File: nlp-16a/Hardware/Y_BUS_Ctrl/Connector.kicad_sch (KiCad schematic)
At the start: 62 parts, among them J1 Conn_02x20_Odd_Even, J2 Conn_02x20_Odd_Even, J3 Conn_02x10_Odd_Even, J4 Conn_02x10_Counter_Clockwise, J5 Screw_Terminal_01x02

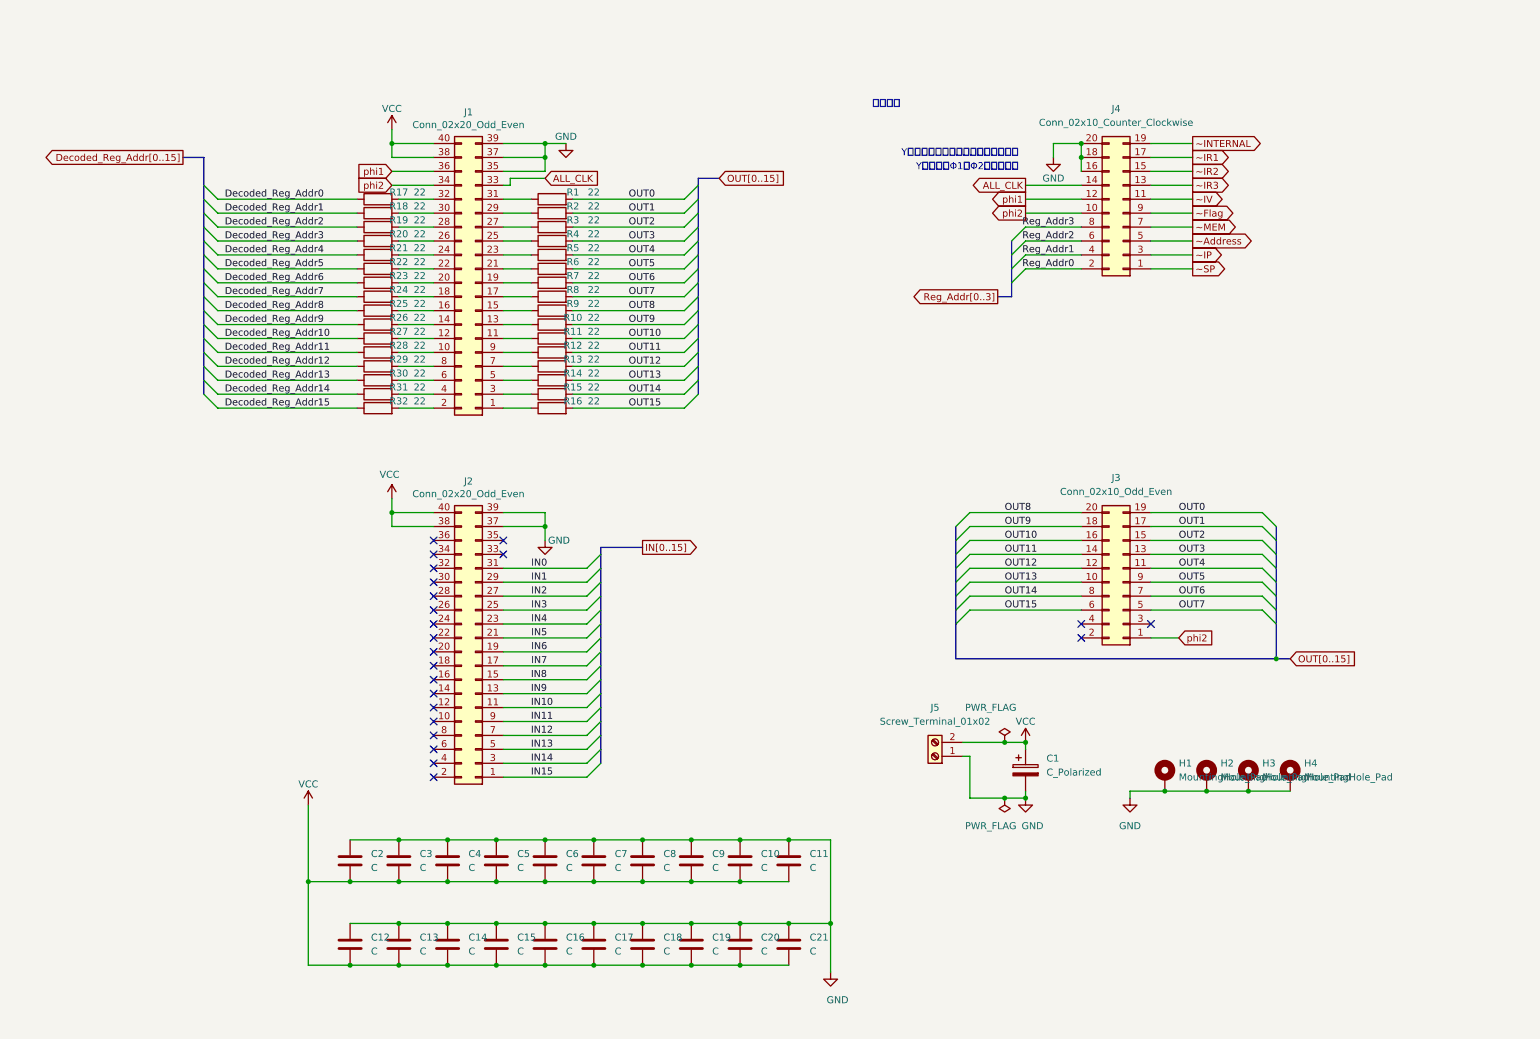
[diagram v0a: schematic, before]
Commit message: Y-BUS制御完成
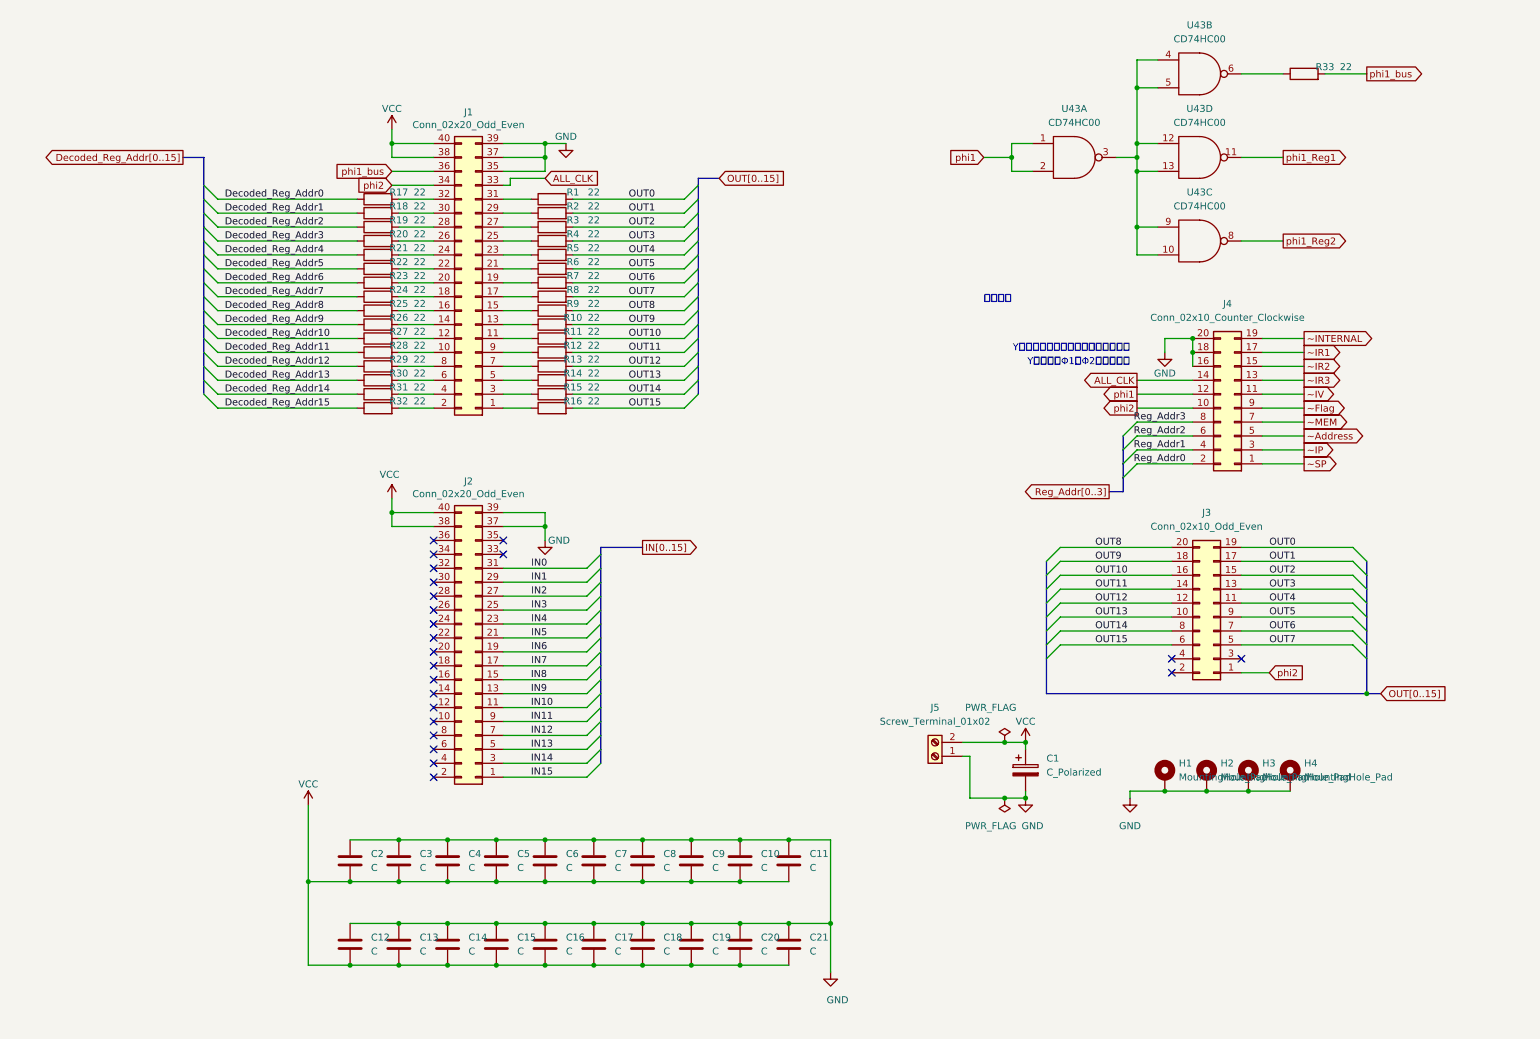
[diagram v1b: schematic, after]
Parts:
- added R33: 22, Resistor_SMD:R_0603_1608Metric_Pad0.98x0.95mm_HandSolder, symbol Device:R
- added U43: CD74HC00, Package_DIP:DIP-14_W7.62mm, symbol CD74HCXX:CD74HC00
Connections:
- net GND: now also U43.7 (GND), U43.7 (GND), U43.7 (GND), U43.7 (GND)
- net VCC: now also U43.14 (VCC), U43.14 (VCC), U43.14 (VCC), U43.14 (VCC)
- net phi1: now also U43.1, U43.2; no longer J1.36 (Pin_36)
- new net: U43.10, U43.12, U43.13, U43.3, U43.4, U43.5, U43.9
- new net: R33.1, U43.6
- new net phi1_Reg1: U43.11
- new net phi1_Reg2: U43.8
- new net phi1_bus: J1.36 (Pin_36), R33.2
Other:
- moved on the sheet: J3, J4

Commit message: Y BUS制御 更新
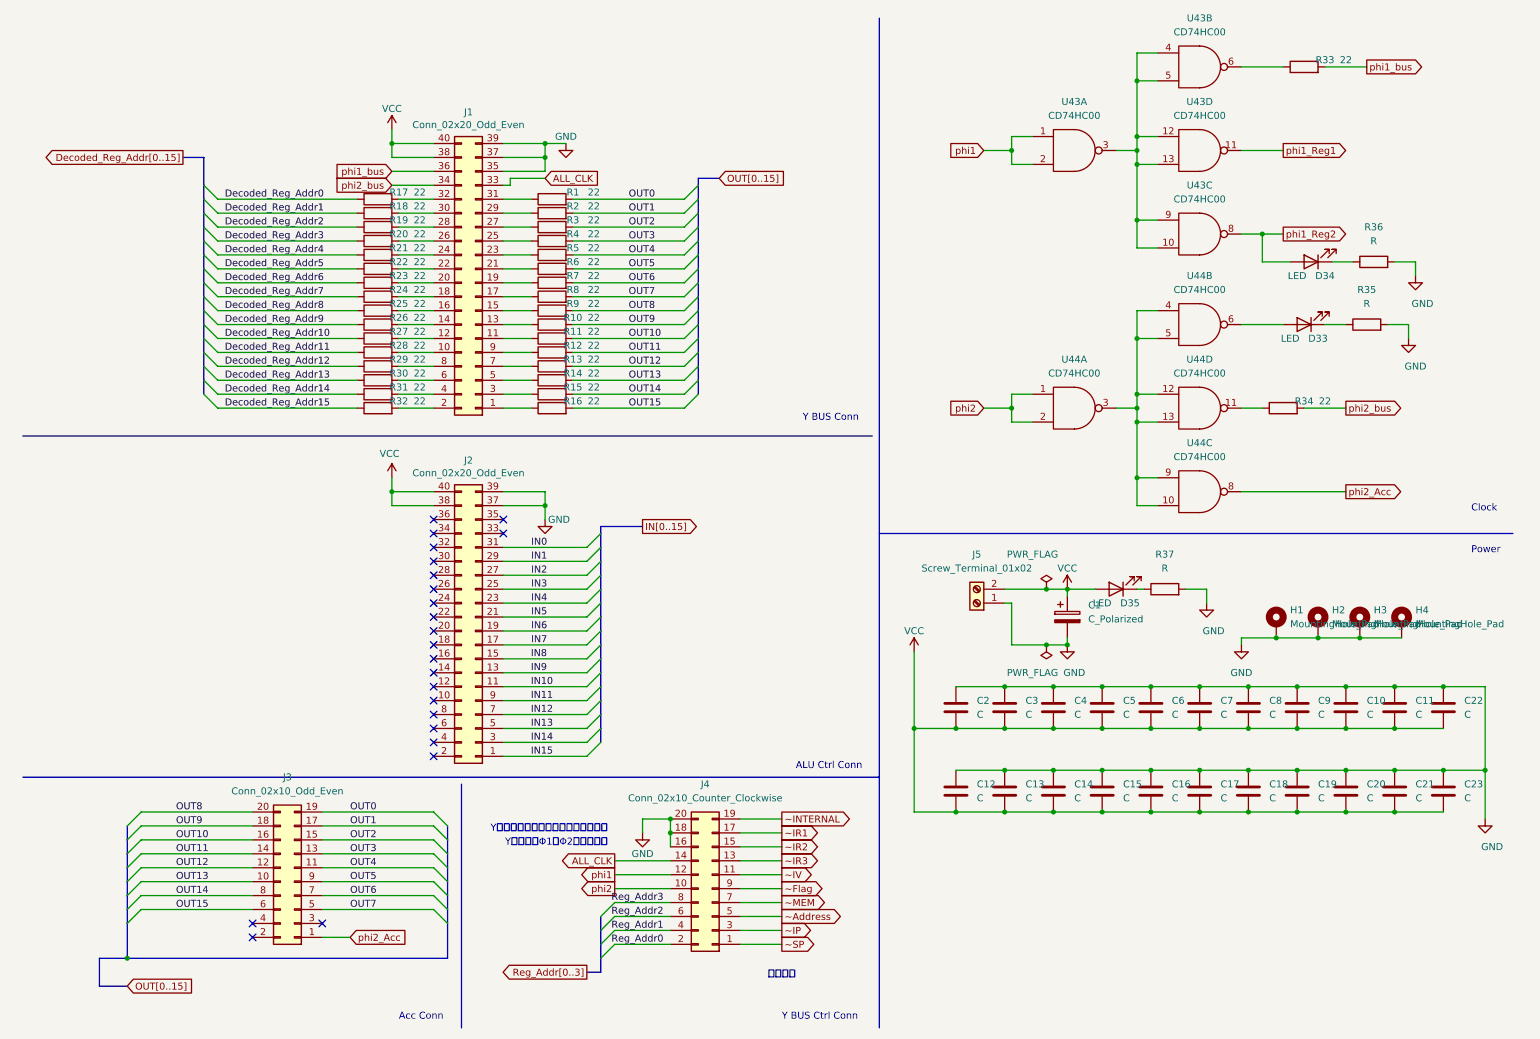
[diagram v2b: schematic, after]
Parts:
- added C22, C23: C, Capacitor_THT:C_Disc_D7.5mm_W2.5mm_P5.00mm, symbol Device:C
- added D33, D34, D35: LED, LED_THT:LED_D3.0mm, symbol Device:LED
- added R34: 22, Resistor_SMD:R_0603_1608Metric_Pad0.98x0.95mm_HandSolder, symbol Device:R
- added R35, R36, R37: R, Resistor_SMD:R_0603_1608Metric_Pad0.98x0.95mm_HandSolder, symbol Device:R
- added U44: CD74HC00, Package_DIP:DIP-14_W7.62mm, symbol CD74HCXX:CD74HC00
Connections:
- net GND: now also C22.1, C23.1, R35.2, R36.2, R37.2, U44.7 (GND), U44.7 (GND), U44.7 (GND), U44.7 (GND)
- net VCC: now also C22.2, C23.2, D35.2 (A), U44.14 (VCC), U44.14 (VCC), U44.14 (VCC), U44.14 (VCC)
- net phi1_Reg2: now also D34.2 (A)
- net phi2: now also U44.1, U44.2; no longer J1.34 (Pin_34), J3.1 (Pin_1)
- new net: R34.1, U44.11
- new net: U44.10, U44.12, U44.13, U44.3, U44.4, U44.5, U44.9
- new net: D33.1 (K), R35.1
- new net: D34.1 (K), R36.1
- new net: D35.1 (K), R37.1
- new net: D33.2 (A), U44.6
- new net phi2_Acc: J3.1 (Pin_1), U44.8
- new net phi2_bus: J1.34 (Pin_34), R34.2
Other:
- note added: "ALU Ctrl Conn"
- note added: "Acc Conn"
- note added: "Clock"
- note added: "Power"
- note added: "Y BUS Conn"
- note added: "Y BUS Ctrl Conn"
- moved on the sheet: C1, C10, C11, C12, C13, C14, C15, C16, C17, C18, C19, C2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
